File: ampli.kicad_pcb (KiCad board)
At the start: 2 copper layers, 110 x 100 mm, 51 parts, among them J2 Conn_01x02, J3 Conn_01x03, Q1 2N2907, Q10 TIP32, Q11 BD138, Q12 TIP31, Q13 2N2222, Q2 2N2907, Q3 2N2907, Q4 2N2222, Q5 2N2222, Q6 2N2907, Q7 2N2907, Q8 BD139, Q9 BD139, U1 Relay_1CT, U2 Jack_Mono

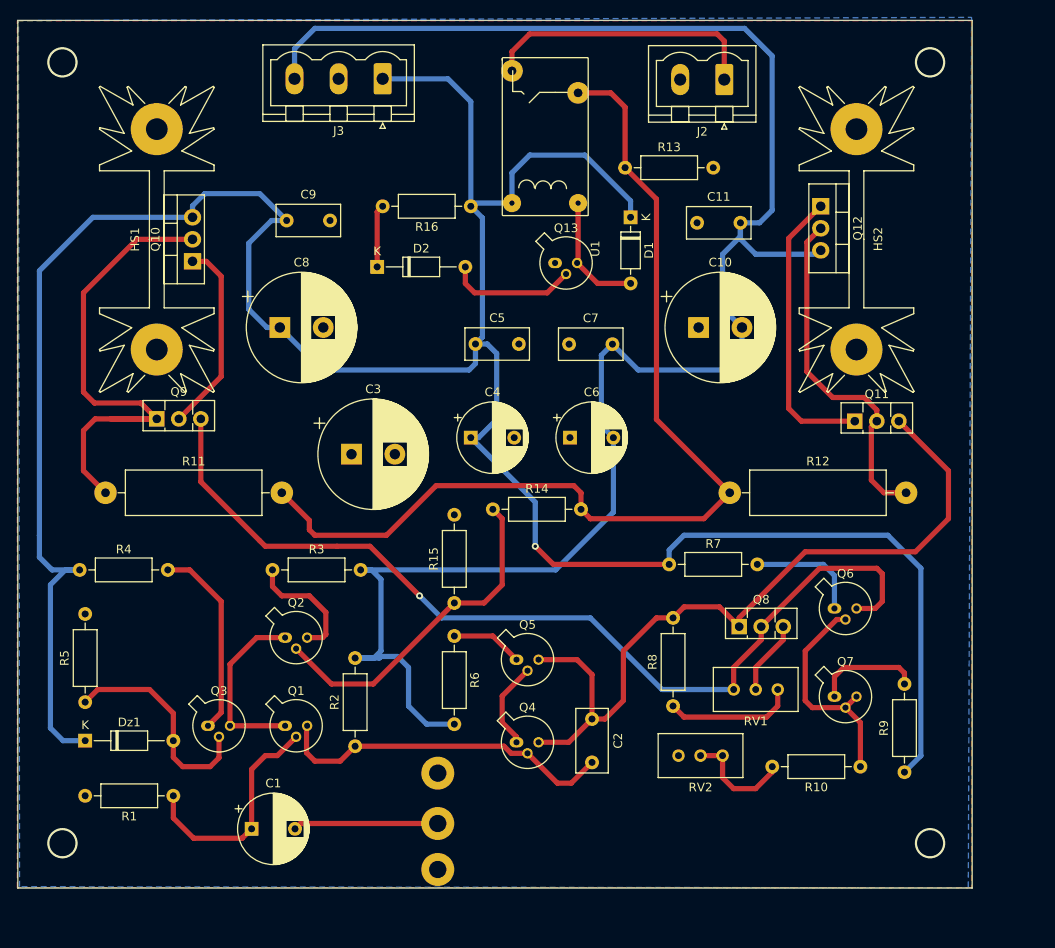
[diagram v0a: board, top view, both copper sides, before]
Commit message: .
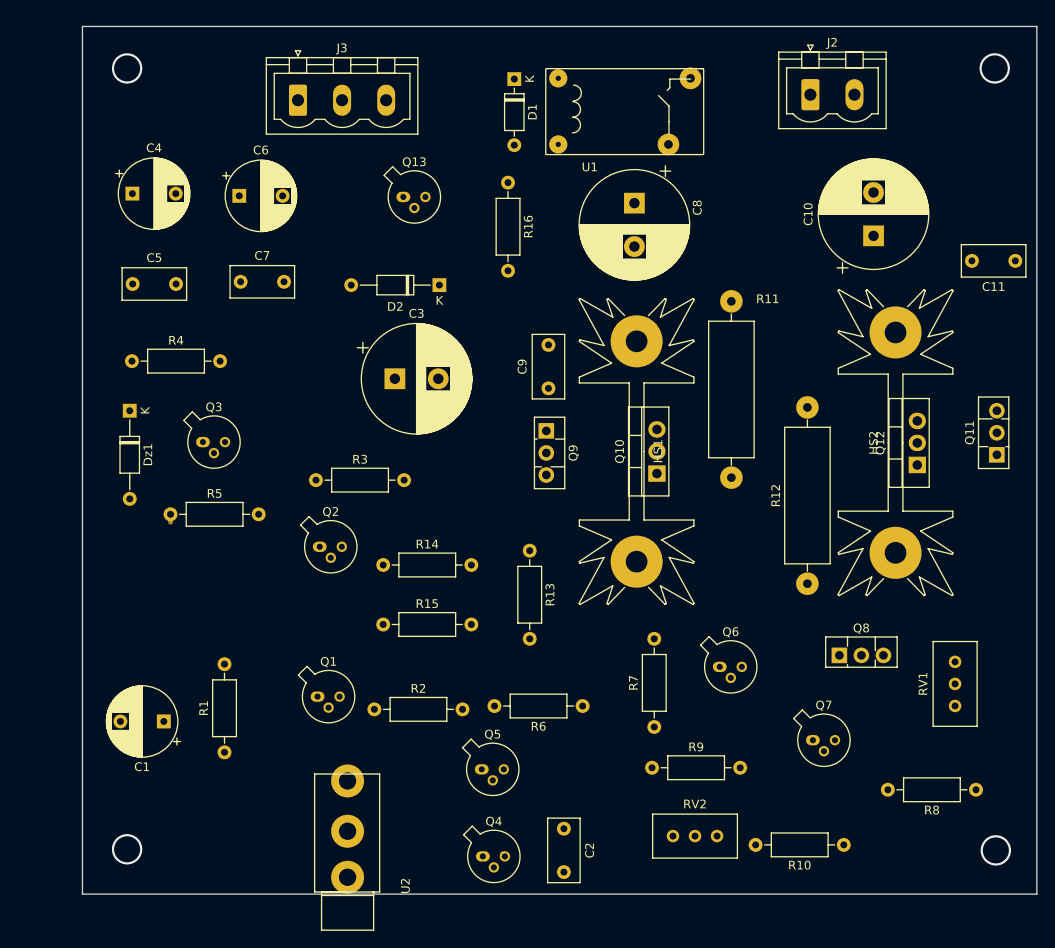
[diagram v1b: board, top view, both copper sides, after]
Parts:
- U2: moved to F.Cu
- moved R11 72.2 mm to (136.3, 77.2), turned to 90 degrees
- moved HS1 60.5 mm to (125.3, 74.2), turned to -90 degrees
- moved Q10 58.8 mm to (127.7, 76.7)
- moved C4 48.1 mm to (67.2, 44.5)
- moved C6 47.2 mm to (79.6, 44.7)
- moved R13 45.5 mm to (113.0, 85.6), turned to -90 degrees
- moved Q9 44.9 mm to (114.9, 71.8), turned to -90 degrees
- moved C8 43.3 mm to (125.1, 45.5), turned to -90 degrees
- moved U1 43.1 mm to (91.3, 48.3), turned to 0 degrees
- moved C5 40.1 mm to (67.3, 54.9)
- moved C7 38.5 mm to (79.7, 54.6)
- moved Dz1 38.4 mm to (66.9, 69.5), turned to -90 degrees
- moved C11 36.9 mm to (169.0, 52.2), turned to 180 degrees
- moved R8 36.2 mm to (164.5, 113.2), turned to 180 degrees
- moved C9 35.8 mm to (115.2, 66.9), turned to 90 degrees
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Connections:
- Q12 pad 1: Net-(Q11-Pad1) -> Net-(Q11-Pad2)
- Q12 pad 2: Net-(Q11-Pad2) -> Net-(Q11-Pad1)
- R12 pad 2: Net-(Q11-Pad2) -> Net-(Q11-Pad1)
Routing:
- net +12V: track 312.9 -> 0.00 mm, vias 1 -> 0
- net -12V: track 212.9 -> 0.00 mm
- net Net-(R11-Pad2): track 116.1 -> 0.00 mm
- net Net-(Q6-Pad3): track 110.6 -> 0.00 mm, vias 1 -> 0
- net Net-(C2-Pad1): track 89.4 -> 0.57 mm
- net Net-(Q10-Pad2): track 58.9 -> 0.00 mm
- net Net-(Q11-Pad2): track 40.0 -> 0.00 mm
- net Net-(C2-Pad2): track 39.9 -> 0.42 mm
- net Net-(Q2-Pad2): track 39.3 -> 0.00 mm
- net Net-(Q11-Pad1): track 33.1 -> 0.00 mm
- net /HP: track 32.3 -> 0.00 mm
- net Net-(C1-Pad1): track 26.5 -> 0.00 mm
- net Net-(Q6-Pad2): track 26.1 -> 0.00 mm
- net Net-(Dz1-Pad2): track 25.5 -> 0.89 mm
- net Net-(Q3-Pad1): track 22.6 -> 0.00 mm
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- removed copper zone on B.Cu, net GND
- removed copper zone on F.Cu, net GND
